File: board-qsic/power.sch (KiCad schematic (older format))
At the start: 25 parts, among them U101 XC7A75T-CSG324, U1201 TPS82085, U1202 TPS82085, U1203 TPS82085, U1204 TPS82085

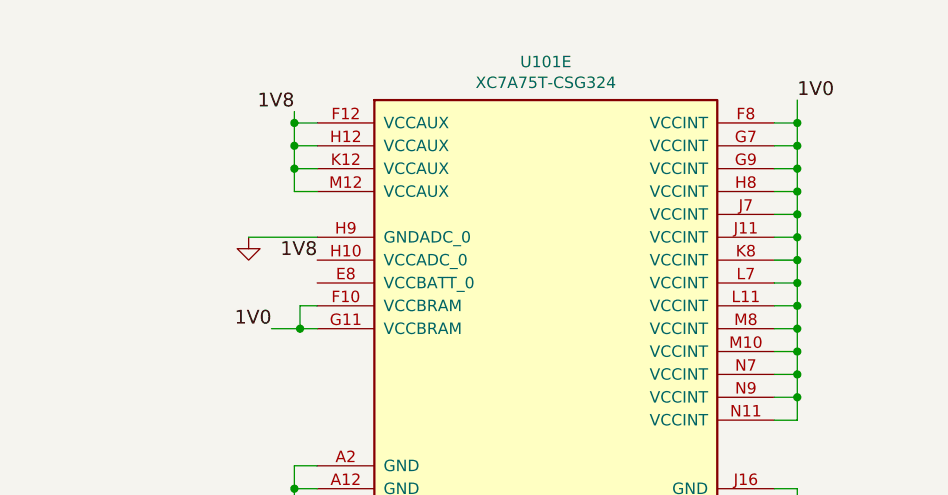
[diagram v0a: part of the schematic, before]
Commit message: Design of prototype is done.  Needs checking before sending out.
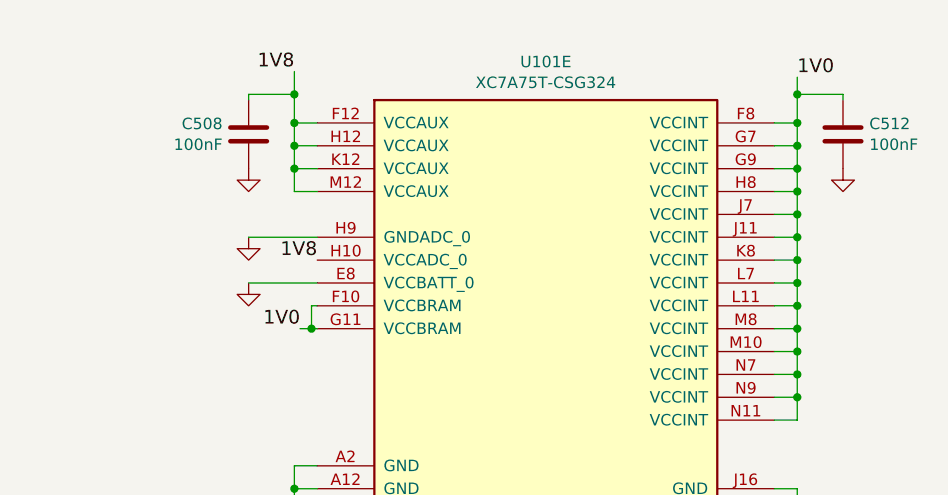
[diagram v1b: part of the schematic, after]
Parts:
- added C508, C512: 100nF, Capacitor_SMD:C_0603_1608Metric, symbol Device:C
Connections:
- net 1V0: now also C512.1
- net 1V8: now also C508.1
- net GND: now also U101.E8 (VCCBATT_0), C508.2, C512.2
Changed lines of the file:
@@
 $Descr A 11000 8500
 encoding utf-8
-Sheet 53 53
+Sheet 5 5
 Title "Power"
-Date "2019-09-30"
+Date "2019-10-07"
 Rev "0.2"
 Comp "QSIC - QBUS Storage & I/O Card"
@@
 $EndDescr
 Wire Wire Line
-	8875 1550 8875 1650
+	8875 1450 8875 1525
 Wire Wire Line
 	8775 1650 8875 1650
@@
 	6675 1950 6775 1950
 Wire Wire Line
-	6675 1600 6675 1650
+	6675 1425 6675 1525
 Wire Wire Line
 	6775 1650 6675 1650
@@
 Text HLabel 1125 1350 0    60   Input ~ 0
 5V
-Text Label 8875 1550 0    60   ~ 0
+Text Label 8875 1450 0    60   ~ 0
 1V0
-Text Label 6675 1600 2    60   ~ 0
+Text Label 6675 1425 2    60   ~ 0
 1V8
 Text HLabel 4050 1500 2    60   Output ~ 0
@@
 $EndComp
 Wire Wire Line
-	6775 2550 6700 2550
-Wire Wire Line
-	6700 2550 6700 2450
-Wire Wire Line
-	6775 2450 6700 2450
-Text Label 6575 2550 2    60   ~ 0
+	6775 2550 6750 2550
+Wire Wire Line
+	6750 2550 6750 2450
+Wire Wire Line
+	6775 2450 6750 2450
+Text Label 6700 2550 2    60   ~ 0
 1V0
 $Comp
@@
 	6475 2150 6775 2150
 Wire Wire Line
-	6575 2550 6700 2550
-Connection ~ 6700 2550
+	6700 2550 6750 2550
+Connection ~ 6750 2550
 $Comp
 L myLib:TPS82085 U1201
@@
 Connection ~ 1225 1500
 Connection ~ 1225 2750
+$Comp
+L Device:C C?
+U 1 1 5DDB3BFE
+P 9075 1700
+AR Path="/5DCB8CA6/5DDB3BFE" Ref="C?"  Part="1"
+AR Path="/5D96DF52/5DDB3BFE" Ref="C512"  Part="1"
+F 0 "C512" H 9190 1746 50  0000 L CNN
+F 1 "100nF" H 9190 1655 50  0000 L CNN
+F 2 "Capacitor_SMD:C_0603_1608Metric" H 9113 1550 50  0001 C CNN
+F 3 "~" H 9075 1700 50  0001 C CNN
+	1    9075 1700
+	1    0    0    -1
+$EndComp
+$Comp
+L Device:C C?
+U 1 1 5DDC711B
+P 6475 1700
+AR Path="/5DCB8CA6/5DDC711B" Ref="C?"  Part="1"
+AR Path="/5D96DF52/5DDC711B" Ref="C508"  Part="1"
+F 0 "C508" H 6361 1746 50  0000 R CNN
+F 1 "100nF" H 6361 1655 50  0000 R CNN
+F 2 "Capacitor_SMD:C_0603_1608Metric" H 6513 1550 50  0001 C CNN
+F 3 "~" H 6475 1700 50  0001 C CNN
+	1    6475 1700
+	1    0    0    -1
+$EndComp
+$Comp
+L power:GND #PWR?
+U 1 1 5DDDA595
+P 6475 1850
+AR Path="/5DCB8CA6/5DCBEACE/5DDDA595" Ref="#PWR?"  Part="1"
+AR Path="/5D96DF52/5DDDA595" Ref="#PWR0148"  Part="1"
+F 0 "#PWR0148" H 6475 1600 50  0001 C CNN
+F 1 "GND" H 6475 1700 50  0001 C CNN
+F 2 "" H 6475 1850 50  0000 C CNN
+F 3 "" H 6475 1850 50  0000 C CNN
+	1    6475 1850
+	1    0    0    -1
+$EndComp
+$Comp
+L power:GND #PWR?
+U 1 1 5DDDD3FE
+P 9075 1850
+AR Path="/5DCB8CA6/5DCBEACE/5DDDD3FE" Ref="#PWR?"  Part="1"
+AR Path="/5D96DF52/5DDDD3FE" Ref="#PWR0149"  Part="1"
+F 0 "#PWR0149" H 9075 1600 50  0001 C CNN
+F 1 "GND" H 9075 1700 50  0001 C CNN
+F 2 "" H 9075 1850 50  0000 C CNN
+F 3 "" H 9075 1850 50  0000 C CNN
+	1    9075 1850
+	1    0    0    -1
+$EndComp
+Wire Wire Line
+	9075 1550 9075 1525
+Wire Wire Line
+	9075 1525 8875 1525
+Connection ~ 8875 1525
+Wire Wire Line
+	8875 1525 8875 1650
+Wire Wire Line
+	6475 1550 6475 1525
+Wire Wire Line
+	6475 1525 6675 1525
+Connection ~ 6675 1525
+Wire Wire Line
+	6675 1525 6675 1650
+$Comp
+L power:GND #PWR?
+U 1 1 5DA43B10
+P 6475 2350
+AR Path="/5DCB8CA6/5DCBEACE/5DA43B10" Ref="#PWR?"  Part="1"
+AR Path="/5D96DF52/5DA43B10" Ref="#PWR?"  Part="1"
+F 0 "#PWR?" H 6475 2100 50  0001 C CNN
+F 1 "GND" H 6475 2200 50  0001 C CNN
+F 2 "" H 6475 2350 50  0000 C CNN
+F 3 "" H 6475 2350 50  0000 C CNN
+	1    6475 2350
+	-1   0    0    -1
+$EndComp
+Wire Wire Line
+	6475 2350 6775 2350
 $EndSCHEMATC
